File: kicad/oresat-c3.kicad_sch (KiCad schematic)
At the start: 0 parts

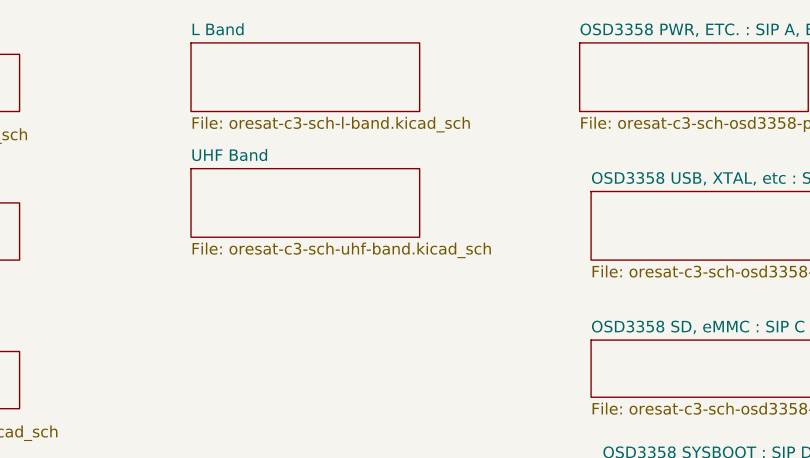
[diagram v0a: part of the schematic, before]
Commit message: Rough draft of watchdog and I2C system schematics.
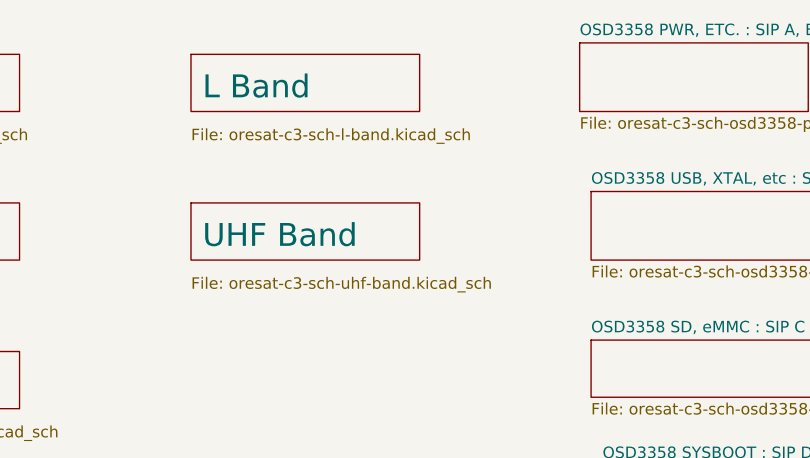
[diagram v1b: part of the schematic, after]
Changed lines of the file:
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@@
 (kicad_sch (version 20230121) (generator eeschema)
   (paper "USLedger")
-  (sheet (at 127 78.74) (size 25.4 7.62) (fields_autoplaced)
+  (sheet (at 127 82.55) (size 25.4 6.35)
     (stroke (width 0.1524) (type solid))
     (fill (color 0 0 0 0.0000))
-    (property "Sheetname" "UHF Band" (at 127 78.0284 0)
-      (effects (font (size 1.27 1.27)) (justify left bottom))
+    (property "Sheetname" "UHF Band" (at 128.27 87.63 0)
+      (effects (font (size 2.54 2.54)) (justify left bottom))
     )
-    (property "Sheetfile" "oresat-c3-sch-uhf-band.kicad_sch" (at 127 86.9446 0)
+    (property "Sheetfile" "oresat-c3-sch-uhf-band.kicad_sch" (at 127 90.7546 0)
       (effects (font (size 1.27 1.27)) (justify left top))
     )
@@
     )
   )
-  (sheet (at 127 64.77) (size 25.4 7.62) (fields_autoplaced)
+  (sheet (at 127 66.04) (size 25.4 6.35)
     (stroke (width 0.1524) (type solid))
     (fill (color 0 0 0 0.0000))
-    (property "Sheetname" "L Band" (at 127 64.0584 0)
-      (effects (font (size 1.27 1.27)) (justify left bottom))
+    (property "Sheetname" "L Band" (at 128.27 71.12 0)
+      (effects (font (size 2.54 2.54)) (justify left bottom))
     )
-    (property "Sheetfile" "oresat-c3-sch-l-band.kicad_sch" (at 127 72.9746 0)
+    (property "Sheetfile" "oresat-c3-sch-l-band.kicad_sch" (at 127 74.2446 0)
       (effects (font (size 1.27 1.27)) (justify left top))
     )
